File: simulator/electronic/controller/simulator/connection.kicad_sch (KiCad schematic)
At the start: 16 parts, among them J1 Conn_01x04_Socket, J1.1 Conn_01x04_Pin, J2 Conn_01x04_Socket, J2.1 Conn_01x04_Pin

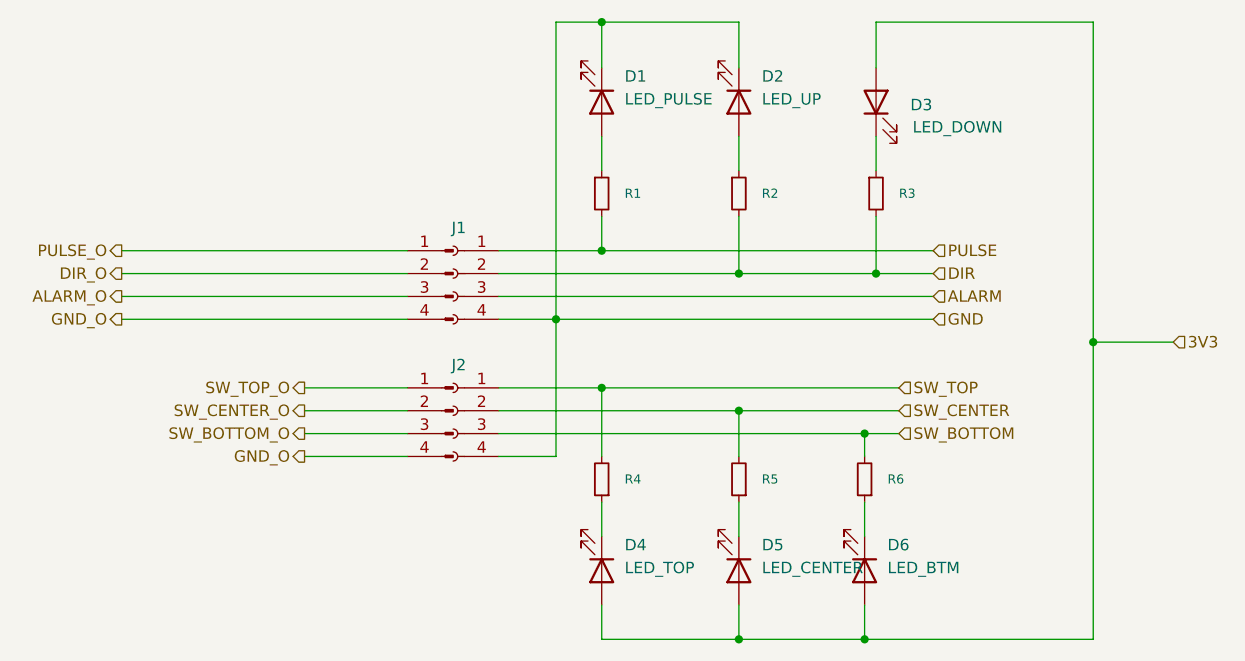
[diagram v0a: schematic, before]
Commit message: update simulator
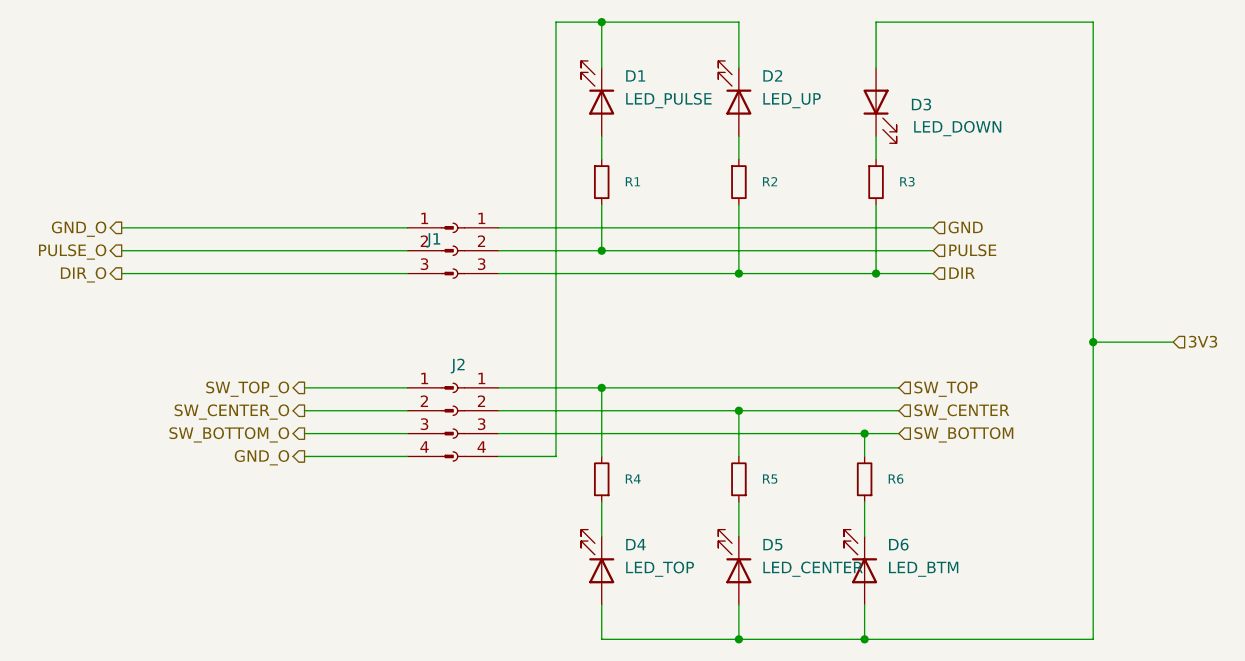
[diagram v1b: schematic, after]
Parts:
- removed J1: Conn_01x04_Socket, Connector_Extra:JST_XH_B4B-XH-A_1x04_P2.54mm_Vertical, symbol Connector:Conn_01x04_Socket
- removed J1.1: Conn_01x04_Pin, symbol Connector:Conn_01x04_Pin
- added J1: Conn_01x03_Socket, Connector_JST:JST_XH_B3B-XH-A_1x03_P2.50mm_Vertical, symbol Connector:Conn_01x03_Socket
- added J1.1: Conn_01x03_Pin, symbol Connector:Conn_01x03_Pin
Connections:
- net DIR: now also J1.3 (Pin_3)
- net DIR_O: now also J1.1.3 (Pin_3)
- net GND: now also J1.1 (Pin_1); no longer D1.1 (K), D2.1 (K), J2.4 (Pin_4)
- net GND_O: now also J1.1.1 (Pin_1)
- net PULSE: now also J1.2 (Pin_2)
- net PULSE_O: now also J1.1.2 (Pin_2)
- new net: D1.1 (K), D2.1 (K), J2.4 (Pin_4)
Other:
- moved on the sheet: R1, R2, R3
